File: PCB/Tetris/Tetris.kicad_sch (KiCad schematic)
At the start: 9 parts, among them J1 Power, J2 PWM, J3 Analog, J4 PWM, J5 Analog, J6 Communication, J7 Digital, M1 RGBMatrix, M2 RGBMatrix

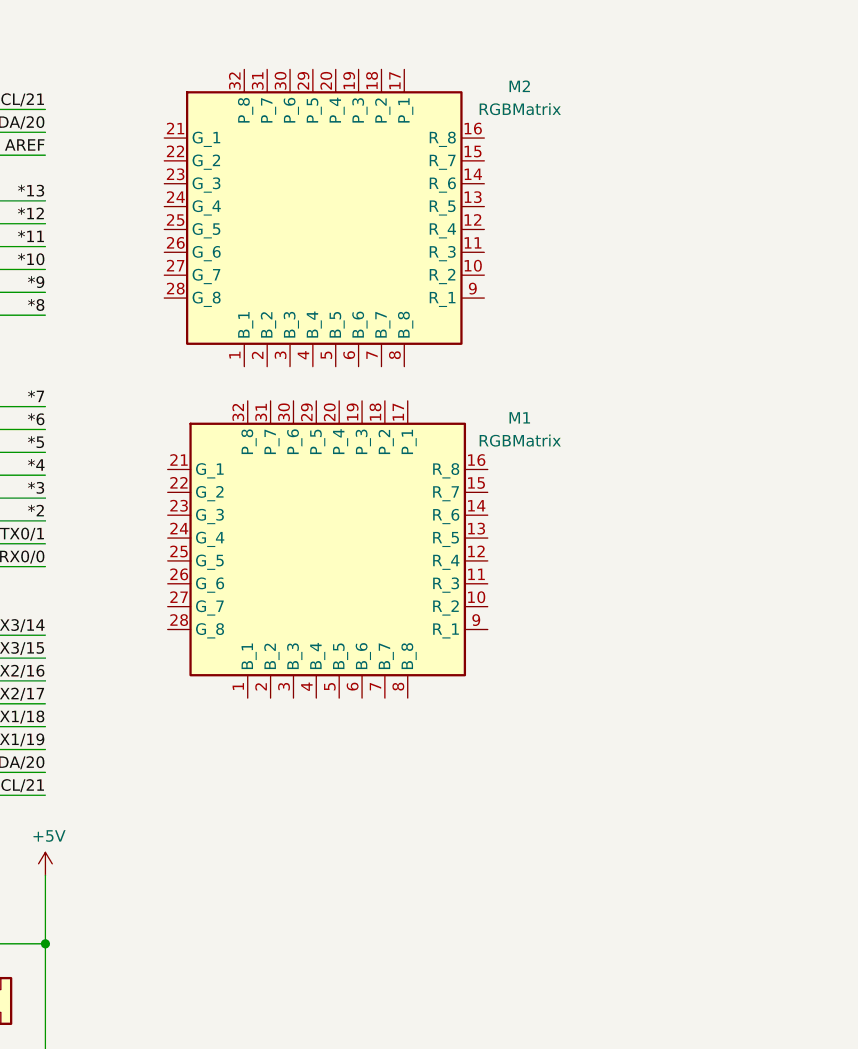
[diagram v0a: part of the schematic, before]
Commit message: something happened
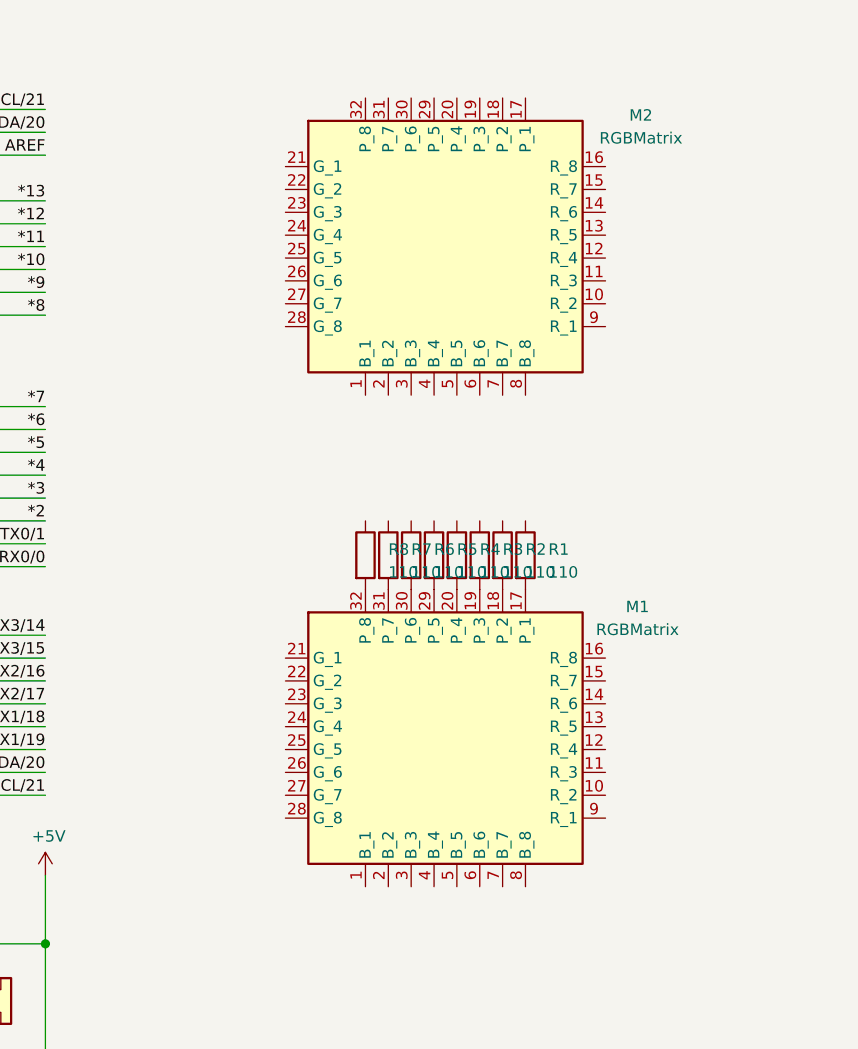
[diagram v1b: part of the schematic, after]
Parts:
- added R1, R2, R3, R4, R5, R6, R7, R8: 110, symbol Device:R
- M1, M2: footprint (none) -> RGBMatrix:RGBMatrix
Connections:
- net at M1.17 (P_1): now also R1.2
- net at M1.18 (P_2): now also R2.2
- net at M1.19 (P_3): now also R3.2
- net at M1.20 (P_4): now also R4.2
- net at M1.29 (P_5): now also R5.2
- net at M1.30 (P_6): now also R6.2
- net at M1.31 (P_7): now also R7.2
- net at M1.32 (P_8): now also R8.2
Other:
- moved on the sheet: M1, M2
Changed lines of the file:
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@@
     )
   )
-  (symbol (lib_id "RGBMatrix:RGBMatrix") (at 105.918 38.735 0) (unit 1)
-    (in_bom yes) (on_board yes) (dnp no) (fields_autoplaced)
-    (property "Reference" "M2" (at 127.635 24.1553 0)
+  (symbol (lib_id "Device:R") (at 113.03 76.2 0) (unit 1)
+    (in_bom yes) (on_board yes) (dnp no) (fields_autoplaced)
+    (property "Reference" "R7" (at 115.57 75.565 0)
+      (effects (font (size 1.27 1.27)) (justify left))
+    )
+    (property "Value" "110" (at 115.57 78.105 0)
+      (effects (font (size 1.27 1.27)) (justify left))
+    )
+    (property "Footprint" "" (at 111.252 76.2 90)
+      (effects (font (size 1.27 1.27)) hide)
+    )
+    (property "Datasheet" "~" (at 113.03 76.2 0)
+      (effects (font (size 1.27 1.27)) hide)
+    )
+    (pin "1")
+    (pin "2")
+    (instances
+      (project "Tetris"
+        (path "/e63e39d7-6ac0-4ffd-8aa3-1841a4541b55"
+          (reference "R7") (unit 1)
+        )
+      )
+    )
+  )
+  (symbol (lib_id "RGBMatrix:RGBMatrix") (at 119.38 41.91 0) (unit 1)
+    (in_bom yes) (on_board yes) (dnp no) (fields_autoplaced)
+    (property "Reference" "M2" (at 141.097 27.3303 0)
       (effects (font (size 1.27 1.27)))
     )
-    (property "Value" "RGBMatrix" (at 127.635 26.6953 0)
+    (property "Value" "RGBMatrix" (at 141.097 29.8703 0)
       (effects (font (size 1.27 1.27)))
     )
-    (property "Footprint" "" (at 105.918 34.925 0)
-      (effects (font (size 1.27 1.27)) hide)
-    )
-    (property "Datasheet" "" (at 105.918 34.925 0)
+    (property "Footprint" "RGBMatrix:RGBMatrix" (at 119.38 38.1 0)
+      (effects (font (size 1.27 1.27)) hide)
+    )
+    (property "Datasheet" "" (at 119.38 38.1 0)
       (effects (font (size 1.27 1.27)) hide)
     )
@@
     )
   )
+  (symbol (lib_id "Device:R") (at 118.11 76.2 0) (unit 1)
+    (in_bom yes) (on_board yes) (dnp no) (fields_autoplaced)
+    (property "Reference" "R5" (at 120.65 75.565 0)
+      (effects (font (size 1.27 1.27)) (justify left))
+    )
+    (property "Value" "110" (at 120.65 78.105 0)
+      (effects (font (size 1.27 1.27)) (justify left))
+    )
+    (property "Footprint" "" (at 116.332 76.2 90)
+      (effects (font (size 1.27 1.27)) hide)
+    )
+    (property "Datasheet" "~" (at 118.11 76.2 0)
+      (effects (font (size 1.27 1.27)) hide)
+    )
+    (pin "1")
+    (pin "2")
+    (instances
+      (project "Tetris"
+        (path "/e63e39d7-6ac0-4ffd-8aa3-1841a4541b55"
+          (reference "R5") (unit 1)
+        )
+      )
+    )
+  )
+  (symbol (lib_id "Device:R") (at 115.57 76.2 0) (unit 1)
+    (in_bom yes) (on_board yes) (dnp no) (fields_autoplaced)
+    (property "Reference" "R6" (at 118.11 75.565 0)
+      (effects (font (size 1.27 1.27)) (justify left))
+    )
+    (property "Value" "110" (at 118.11 78.105 0)
+      (effects (font (size 1.27 1.27)) (justify left))
+    )
+    (property "Footprint" "" (at 113.792 76.2 90)
+      (effects (font (size 1.27 1.27)) hide)
+    )
+    (property "Datasheet" "~" (at 115.57 76.2 0)
+      (effects (font (size 1.27 1.27)) hide)
+    )
+    (pin "1")
+    (pin "2")
+    (instances
+      (project "Tetris"
+        (path "/e63e39d7-6ac0-4ffd-8aa3-1841a4541b55"
+          (reference "R6") (unit 1)
+        )
+      )
+    )
+  )
   (symbol (lib_id "power:VCC") (at 26.67 26.67 0) (unit 1)
     (in_bom yes) (on_board yes) (dnp no)
@@
     )
   )
-  (symbol (lib_id "RGBMatrix:RGBMatrix") (at 106.299 75.565 0) (unit 1)
-    (in_bom yes) (on_board yes) (dnp no) (fields_autoplaced)
-    (property "Reference" "M1" (at 127.635 60.9853 0)
+  (symbol (lib_id "Device:R") (at 128.27 76.2 0) (unit 1)
+    (in_bom yes) (on_board yes) (dnp no) (fields_autoplaced)
+    (property "Reference" "R1" (at 130.81 75.565 0)
+      (effects (font (size 1.27 1.27)) (justify left))
+    )
+    (property "Value" "110" (at 130.81 78.105 0)
+      (effects (font (size 1.27 1.27)) (justify left))
+    )
+    (property "Footprint" "" (at 126.492 76.2 90)
+      (effects (font (size 1.27 1.27)) hide)
+    )
+    (property "Datasheet" "~" (at 128.27 76.2 0)
+      (effects (font (size 1.27 1.27)) hide)
+    )
+    (pin "1")
+    (pin "2")
+    (instances
+      (project "Tetris"
+        (path "/e63e39d7-6ac0-4ffd-8aa3-1841a4541b55"
+          (reference "R1") (unit 1)
+        )
+      )
+    )
+  )
+  (symbol (lib_id "Device:R") (at 120.65 76.2 0) (unit 1)
+    (in_bom yes) (on_board yes) (dnp no) (fields_autoplaced)
+    (property "Reference" "R4" (at 123.19 75.565 0)
+      (effects (font (size 1.27 1.27)) (justify left))
+    )
+    (property "Value" "110" (at 123.19 78.105 0)
+      (effects (font (size 1.27 1.27)) (justify left))
+    )
+    (property "Footprint" "" (at 118.872 76.2 90)
+      (effects (font (size 1.27 1.27)) hide)
+    )
+    (property "Datasheet" "~" (at 120.65 76.2 0)
+      (effects (font (size 1.27 1.27)) hide)
+    )
+    (pin "1")
+    (pin "2")
+    (instances
+      (project "Tetris"
+        (path "/e63e39d7-6ac0-4ffd-8aa3-1841a4541b55"
+          (reference "R4") (unit 1)
+        )
+      )
+    )
+  )
+  (symbol (lib_id "Device:R") (at 123.19 76.2 0) (unit 1)
+    (in_bom yes) (on_board yes) (dnp no) (fields_autoplaced)
+    (property "Reference" "R3" (at 125.73 75.565 0)
+      (effects (font (size 1.27 1.27)) (justify left))
+    )
+    (property "Value" "110" (at 125.73 78.105 0)
+      (effects (font (size 1.27 1.27)) (justify left))
+    )
+    (property "Footprint" "" (at 121.412 76.2 90)
+      (effects (font (size 1.27 1.27)) hide)
+    )
+    (property "Datasheet" "~" (at 123.19 76.2 0)
+      (effects (font (size 1.27 1.27)) hide)
+    )
+    (pin "1")
+    (pin "2")
+    (instances
+      (project "Tetris"
+        (path "/e63e39d7-6ac0-4ffd-8aa3-1841a4541b55"
+          (reference "R3") (unit 1)
+        )
+      )
+    )
+  )
+  (symbol (lib_id "Device:R") (at 125.73 76.2 0) (unit 1)
+    (in_bom yes) (on_board yes) (dnp no) (fields_autoplaced)
+    (property "Reference" "R2" (at 128.27 75.565 0)
+      (effects (font (size 1.27 1.27)) (justify left))
+    )
+    (property "Value" "110" (at 128.27 78.105 0)
+      (effects (font (size 1.27 1.27)) (justify left))
+    )
+    (property "Footprint" "" (at 123.952 76.2 90)
+      (effects (font (size 1.27 1.27)) hide)
+    )
+    (property "Datasheet" "~" (at 125.73 76.2 0)
+      (effects (font (size 1.27 1.27)) hide)
+    )
+    (pin "1")
+    (pin "2")
+    (instances
+      (project "Tetris"
+        (path "/e63e39d7-6ac0-4ffd-8aa3-1841a4541b55"
+          (reference "R2") (unit 1)
+        )
+      )
+    )
+  )
+  (symbol (lib_id "RGBMatrix:RGBMatrix") (at 119.38 96.52 0) (unit 1)
+    (in_bom yes) (on_board yes) (dnp no) (fields_autoplaced)
+    (property "Reference" "M1" (at 140.716 81.9403 0)
       (effects (font (size 1.27 1.27)))
     )
-    (property "Value" "RGBMatrix" (at 127.635 63.5253 0)
+    (property "Value" "RGBMatrix" (at 140.716 84.4803 0)
       (effects (font (size 1.27 1.27)))
     )
-    (property "Footprint" "" (at 106.299 71.755 0)
-      (effects (font (size 1.27 1.27)) hide)
-    )
-    (property "Datasheet" "" (at 106.299 71.755 0)
+    (property "Footprint" "RGBMatrix:RGBMatrix" (at 119.38 92.71 0)
+      (effects (font (size 1.27 1.27)) hide)
+    )
+    (property "Datasheet" "" (at 119.38 92.71 0)
       (effects (font (size 1.27 1.27)) hide)
     )
@@
         )
       )
+    )
+  )
+  (symbol (lib_id "Device:R") (at 110.49 76.2 0) (unit 1)
+    (in_bom yes) (on_board yes) (dnp no) (fields_autoplaced)
+    (property "Reference" "R8" (at 113.03 75.565 0)
+      (effects (font (size 1.27 1.27)) (justify left))
+    )
+    (property "Value" "110" (at 113.03 78.105 0)
+      (effects (font (size 1.27 1.27)) (justify left))
+    )
+    (property "Footprint" "" (at 108.712 76.2 90)
+      (effects (font (size 1.27 1.27)) hide)
+    )
+    (property "Datasheet" "~" (at 110.49 76.2 0)
+      (effects (font (size 1.27 1.27)) hide)
+    )
+    (pin "1")
+    (pin "2")
+    (instances
+      (project "Tetris"
+        (path "/e63e39d7-6ac0-4ffd-8aa3-1841a4541b55"
+          (reference "R8") (unit 1)
+        )
+      )

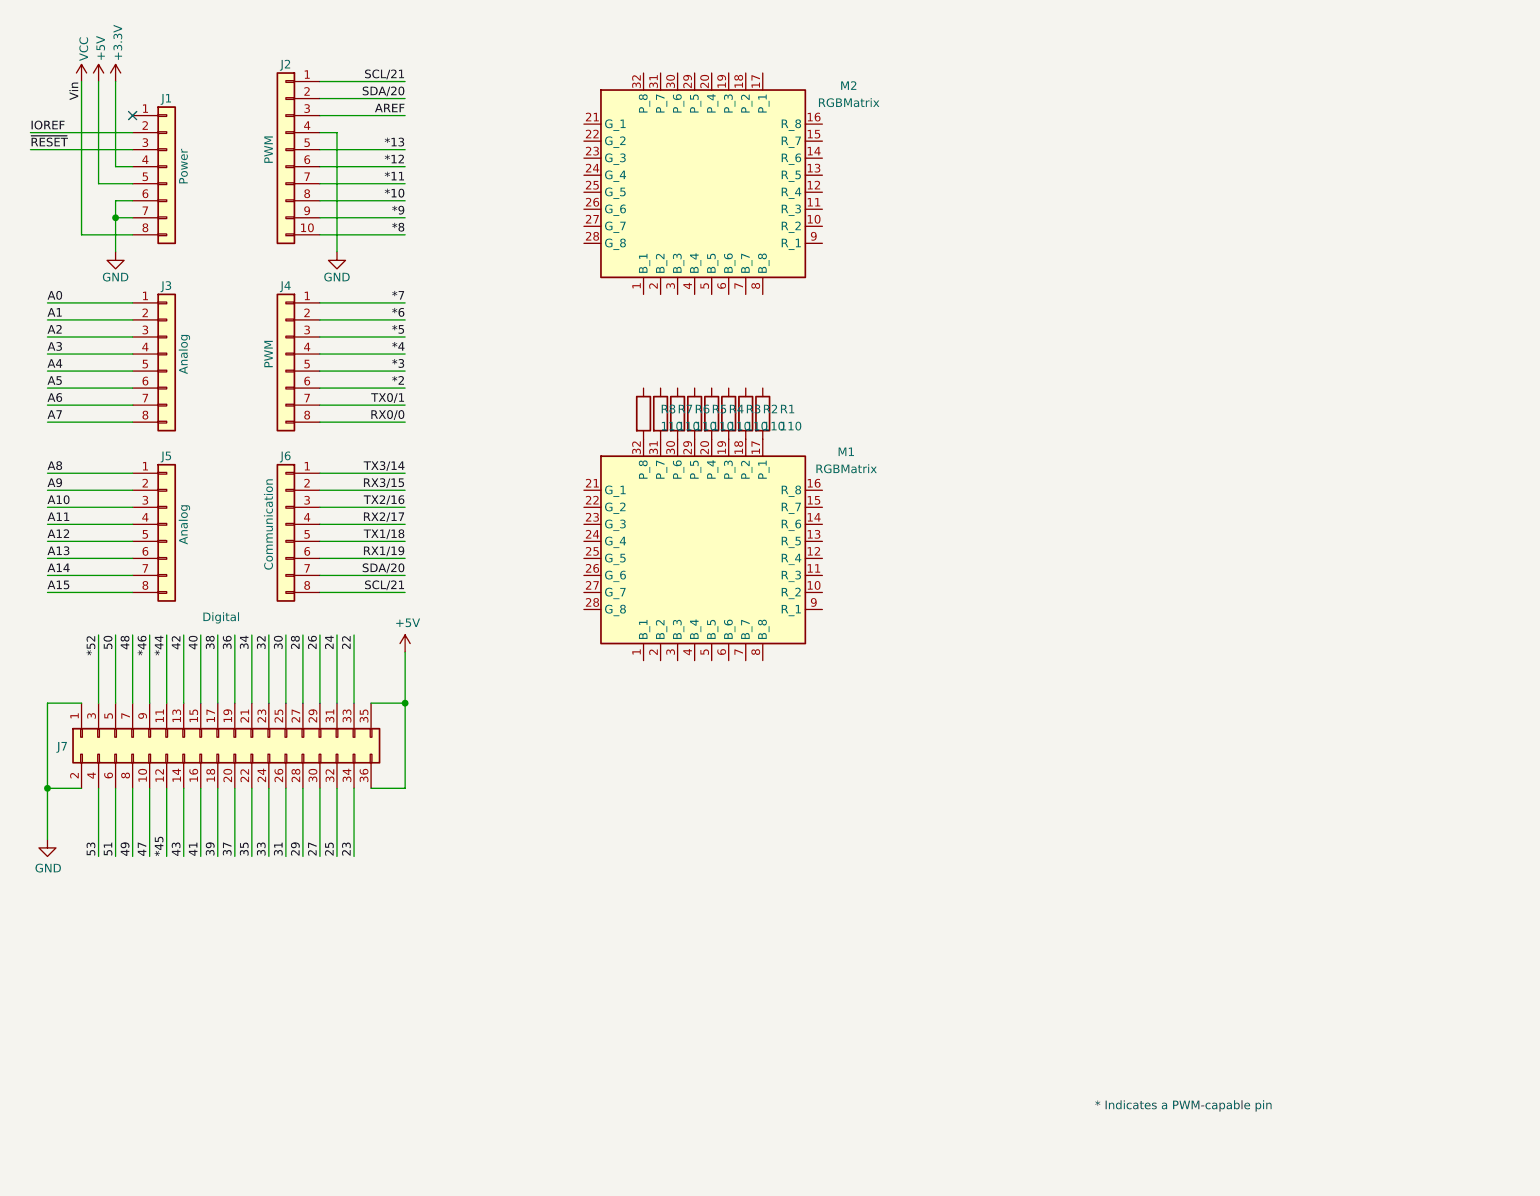
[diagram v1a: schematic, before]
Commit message: Schematics and sync
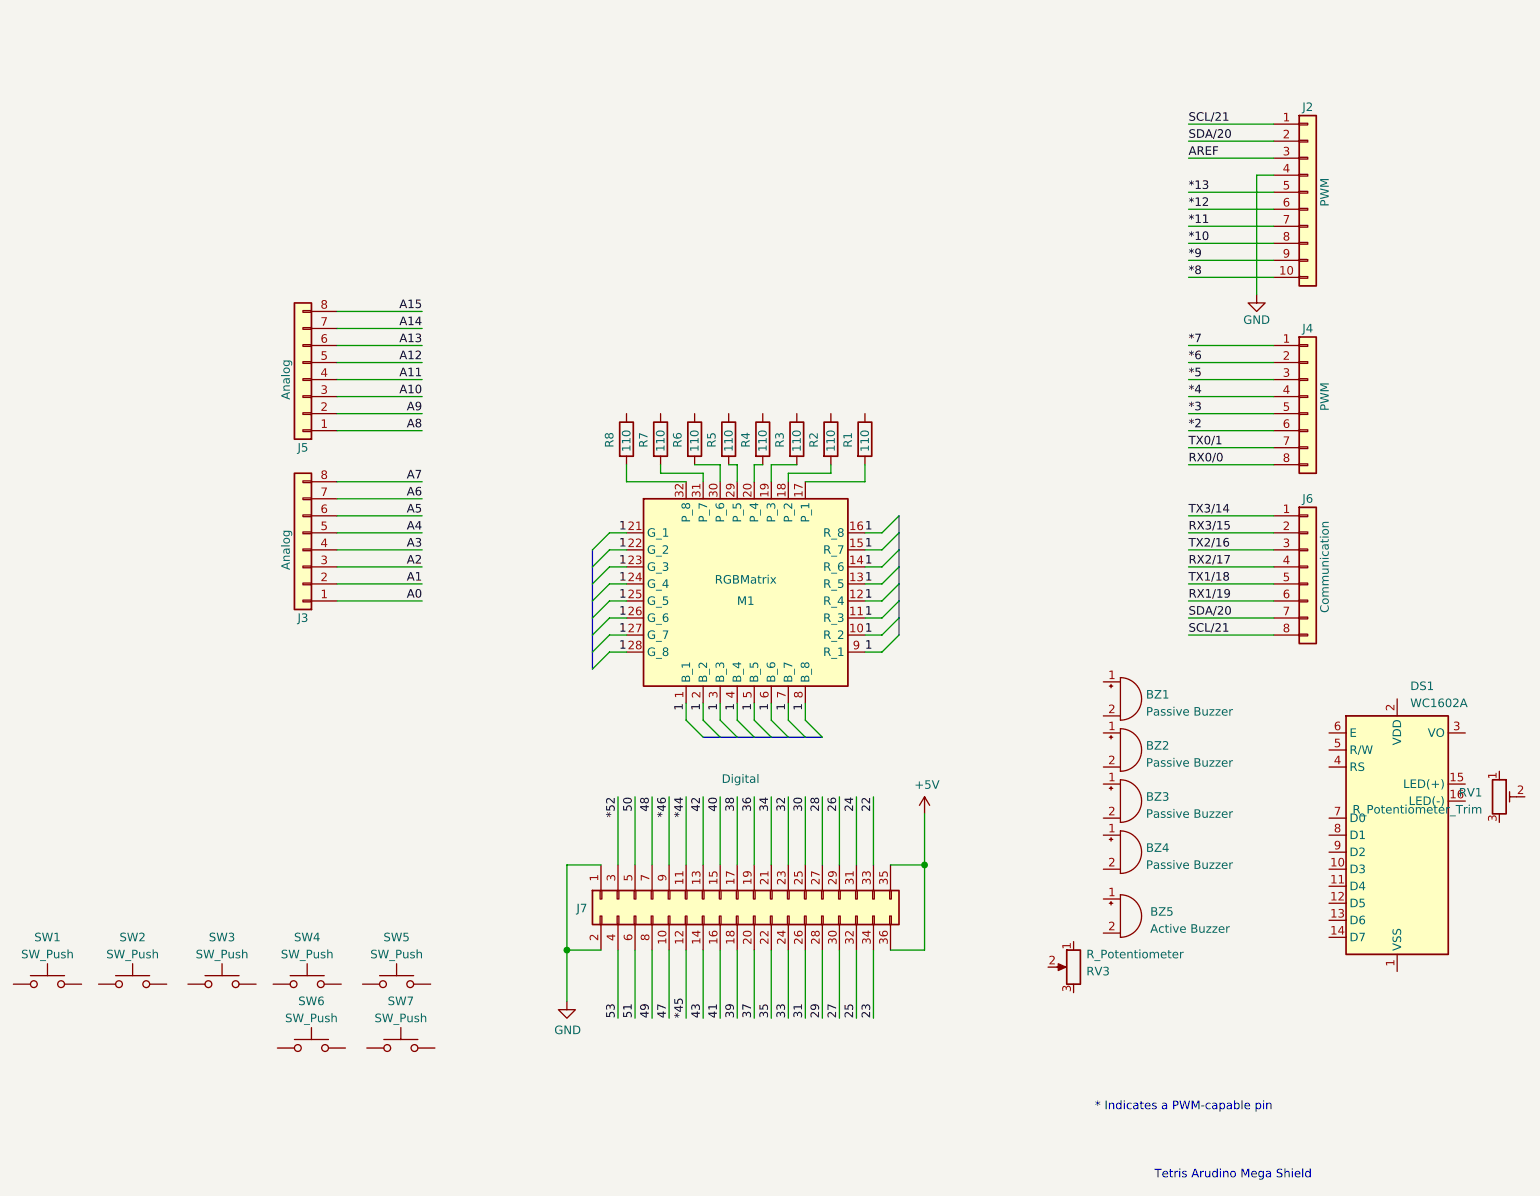
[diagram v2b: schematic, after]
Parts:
- removed J1: Power, Connector_PinSocket_2.54mm:PinSocket_1x08_P2.54mm_Vertical, symbol Connector_Generic:Conn_01x08
- removed M2: RGBMatrix, RGBMatrix:RGBMatrix, symbol RGBMatrix:RGBMatrix
- added BZ1, BZ2, BZ3, BZ4: Passive Buzzer, symbol Device:Buzzer
- added BZ5: Active Buzzer, symbol Device:Buzzer
- added DS1: WC1602A, Display:WC1602A, symbol Display_Character:WC1602A
- added RV1: R_Potentiometer_Trim, symbol Device:R_Potentiometer_Trim
- added RV3: R_Potentiometer, symbol Device:R_Potentiometer
- added SW1, SW2, SW3, SW4, SW5, SW6, SW7: SW_Push, symbol Switch:SW_Push
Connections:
- net 1: now reaches M1.1 (B_1)
- net 1: now also M1.10 (R_2), M1.11 (R_3), M1.12 (R_4), M1.13 (R_5), M1.14 (R_6), M1.15 (R_7), M1.16 (R_8), M1.2 (B_2), M1.21 (G_1), M1.22 (G_2), M1.23 (G_3), M1.24 (G_4), M1.25 (G_5), M1.26 (G_6), M1.27 (G_7), M1.28 (G_8), M1.3 (B_3), M1.4 (B_4), M1.5 (B_5), M1.6 (B_6), M1.7 (B_7), M1.8 (B_8), M1.9 (R_1)
- no-connect marks 1 -> 0
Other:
- note added: "Tetris Arudino Mega Shield"
- moved on the sheet: J2, J3, J4, J5, J6, J7, M1
